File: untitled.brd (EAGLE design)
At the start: 92.8 x 83.4 mm, 176 parts, among them IC1 MCP23017SS, IC4 MCP23017SS, K2 351, Q1 S9013, U49 PC817X2NIP0F, X1 MSTBA12, X2 MSTBA12, X5 MSTBA3, X6 MSTBA3, X7 MSTBA2, X8 MSTBA2

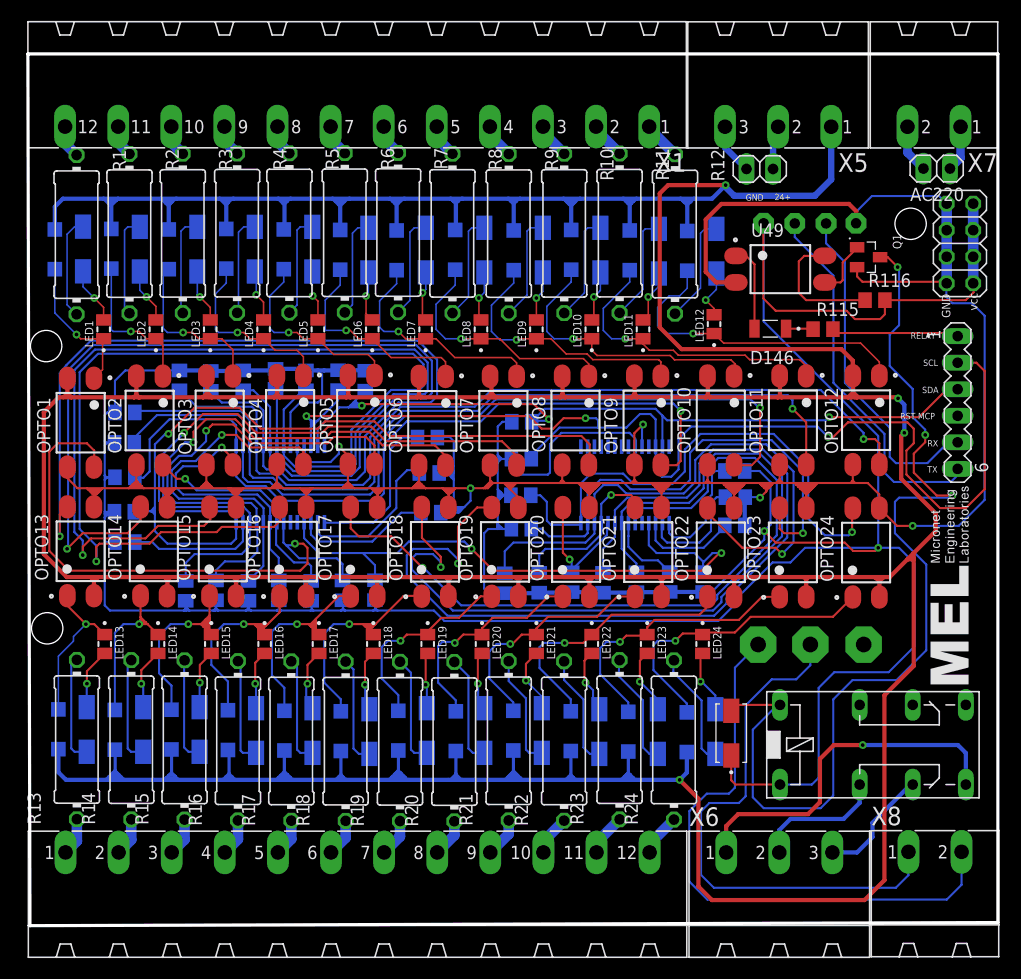
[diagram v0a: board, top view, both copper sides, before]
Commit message: revisi board
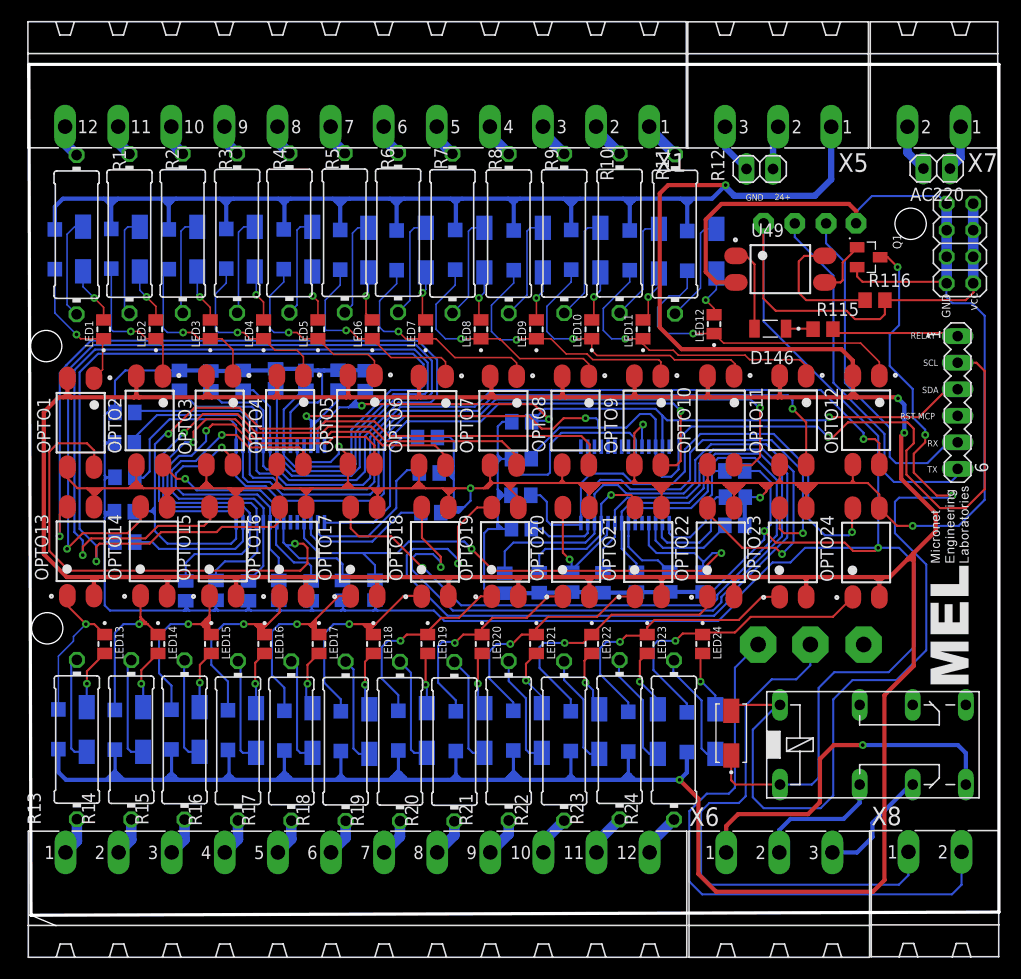
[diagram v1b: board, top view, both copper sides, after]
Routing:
- net COMM: track 674.1 -> 672.8 mm
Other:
- board size 92.8 x 83.4 mm -> 92.8 x 82.4 mm
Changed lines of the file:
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@@
 <setting verticaltext="up"/>
 </settings>
-<grid distance="0.75" unitdist="mil" unit="mm" style="lines" multiple="1" display="yes" altdistance="5" altunitdist="mil" altunit="mm"/>
+<grid distance="0.1" unitdist="mm" unit="mm" style="lines" multiple="1" display="yes" altdistance="5" altunitdist="mil" altunit="mm"/>
 <layers>
 <layer number="1" name="Top" color="4" fill="1" visible="yes" active="yes"/>
@@
 <board>
 <plain>
-<wire x1="0.55" y1="-0.25" x2="93.15" y2="0.05" width="0.3048" layer="20"/>
-<wire x1="93.15" y1="0.05" x2="93.15" y2="83.15" width="0.3048" layer="20"/>
-<wire x1="93.15" y1="83.15" x2="0.35" y2="83.15" width="0.3048" layer="20"/>
-<wire x1="0.35" y1="83.15" x2="0.55" y2="-0.25" width="0.3048" layer="20"/>
-<wire x1="0.55" y1="-0.25" x2="3.05" y2="-0.25" width="0" layer="20"/>
+<wire x1="0.65" y1="0.75" x2="93.25" y2="1.05" width="0.3048" layer="20"/>
+<wire x1="93.25" y1="1.05" x2="93.25" y2="82.15" width="0.3048" layer="20"/>
+<wire x1="93.25" y1="82.15" x2="0.45" y2="82.15" width="0.3048" layer="20"/>
+<wire x1="0.45" y1="82.15" x2="0.65" y2="0.75" width="0.3048" layer="20"/>
+<wire x1="0.65" y1="0.75" x2="3.05" y2="-0.25" width="0" layer="20"/>
 <circle x="84.8" y="66.9" radius="1.5" width="0.0762" layer="20"/>
 <circle x="2.1" y="55.2" radius="1.5" width="0.0762" layer="20"/>
@@
 <wire x1="85.1" y1="24.6" x2="82.3" y2="21.8" width="0.4064" layer="1"/>
 <wire x1="82.3" y1="21.8" x2="82.3" y2="4.10525" width="0.4064" layer="1"/>
-<wire x1="82.3" y1="4.10525" x2="80.39475" y2="2.2" width="0.4064" layer="1"/>
-<wire x1="80.39475" y1="2.2" x2="65.8" y2="2.2" width="0.4064" layer="1"/>
-<wire x1="65.8" y1="2.2" x2="64.5" y2="3.5" width="0.4064" layer="1"/>
-<wire x1="64.5" y1="3.5" x2="64.5" y2="11.9" width="0.4064" layer="1"/>
+<wire x1="82.3" y1="4.10525" x2="81.19475" y2="3" width="0.4064" layer="1"/>
+<wire x1="81.19475" y1="3" x2="66.2" y2="3" width="0.4064" layer="1"/>
+<wire x1="66.2" y1="3" x2="64.5" y2="4.7" width="0.4064" layer="1"/>
+<wire x1="64.5" y1="4.7" x2="64.5" y2="11.9" width="0.4064" layer="1"/>
 <wire x1="64.5" y1="11.9" x2="62.7" y2="13.7" width="0.4064" layer="1"/>
 <wire x1="85.1" y1="35.4" x2="85.1" y2="35.052" width="0.2" layer="1"/>
@@
 <contactref element="X8" pad="1"/>
 <wire x1="84.5947" y1="6.81355" x2="84.5947" y2="4.5847" width="0.2" layer="16"/>
-<wire x1="84.5947" y1="4.5847" x2="83.38185" y2="3.37185" width="0.2" layer="16"/>
-<wire x1="83.38185" y1="3.37185" x2="65.9892" y2="3.37185" width="0.2" layer="16"/>
-<wire x1="65.9892" y1="3.37185" x2="64.75095" y2="4.6101" width="0.2" layer="16"/>
+<wire x1="84.5947" y1="4.5847" x2="83.68185" y2="3.67185" width="0.2" layer="16"/>
+<wire x1="83.68185" y1="3.67185" x2="65.6892" y2="3.67185" width="0.2" layer="16"/>
+<wire x1="65.6892" y1="3.67185" x2="64.75095" y2="4.6101" width="0.2" layer="16"/>
 <wire x1="64.75095" y1="4.6101" x2="64.75095" y2="10.68705" width="0.2" layer="16"/>
 <wire x1="64.75095" y1="10.68705" x2="65.55105" y2="11.48715" width="0.2" layer="16"/>
@@
 <contactref element="X8" pad="2"/>
 <wire x1="89.6747" y1="6.81355" x2="89.6747" y2="3.66395" width="0.2" layer="16"/>
-<wire x1="89.6747" y1="3.66395" x2="88.25865" y2="2.2479" width="0.2" layer="16"/>
-<wire x1="88.25865" y1="2.2479" x2="65.36055" y2="2.2479" width="0.2" layer="16"/>
-<wire x1="65.36055" y1="2.2479" x2="63.627" y2="3.98145" width="0.2" layer="16"/>
+<wire x1="89.6747" y1="3.66395" x2="88.75865" y2="2.7479" width="0.2" layer="16"/>
+<wire x1="88.75865" y1="2.7479" x2="64.86055" y2="2.7479" width="0.2" layer="16"/>
+<wire x1="64.86055" y1="2.7479" x2="63.627" y2="3.98145" width="0.2" layer="16"/>
 <wire x1="63.627" y1="3.98145" x2="63.627" y2="10.7061" width="0.2" layer="16"/>
 <wire x1="63.627" y1="10.7061" x2="65.3034" y2="12.3825" width="0.2" layer="16"/>

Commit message: revisi .brd
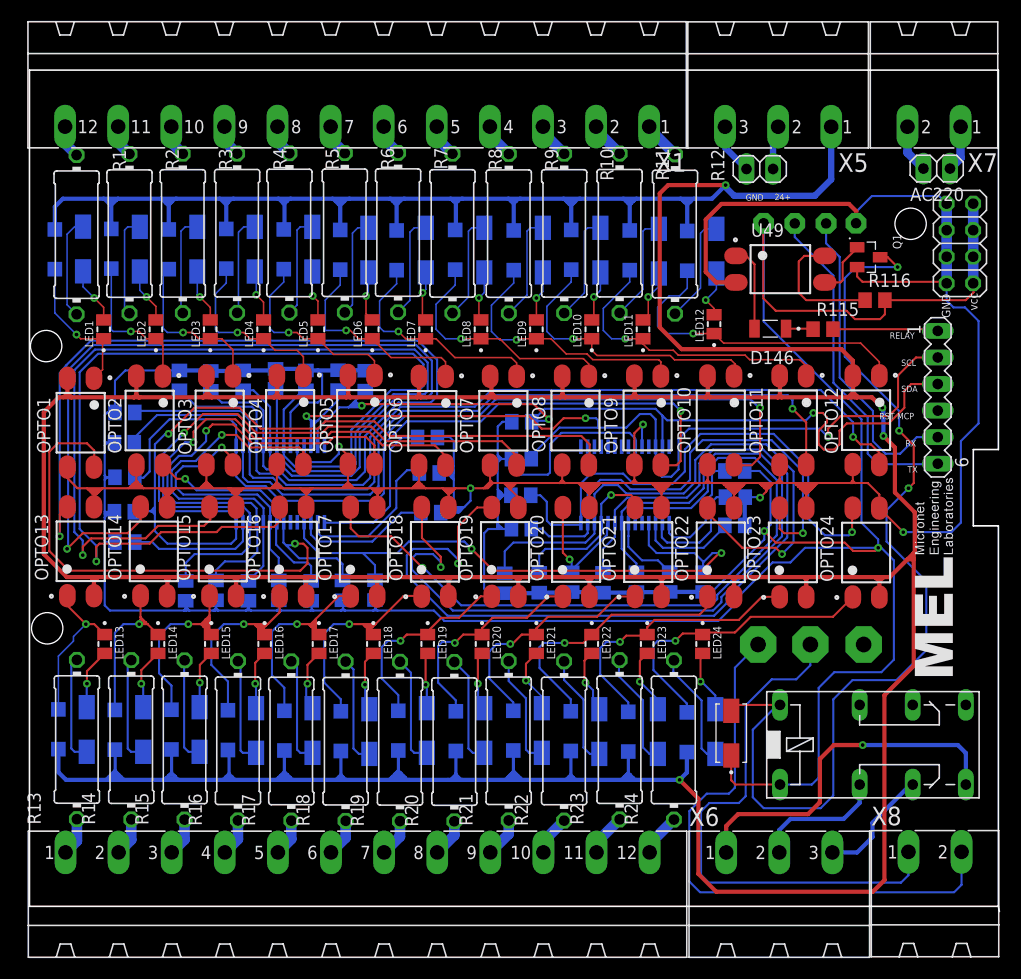
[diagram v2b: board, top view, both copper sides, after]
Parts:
- moved SV2 1.96 mm to (87.4, 50.3)
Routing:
- net SCL: track 115.9 -> 94.1 mm
- net SDA: track 78.2 -> 83.7 mm
- net TX: track 35.6 -> 32.1 mm
- net COMM: track 672.8 -> 669.4 mm
- net VCC: track 363.7 -> 360.6 mm
- net RX: track 32.4 -> 30.0 mm
- net RELAY: track 12.2 -> 10.7 mm
- net N$101: track 93.4 -> 92.2 mm
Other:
- board size 92.8 x 82.4 mm -> 92.8 x 80.5 mm
